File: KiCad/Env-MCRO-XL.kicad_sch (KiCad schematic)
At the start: 49 parts, among them SW1 RotaryEncoder_Switch, SW2 RotaryEncoder_Switch, SW3 RotaryEncoder_Switch, SW4 RotaryEncoder_Switch, U1 Pico

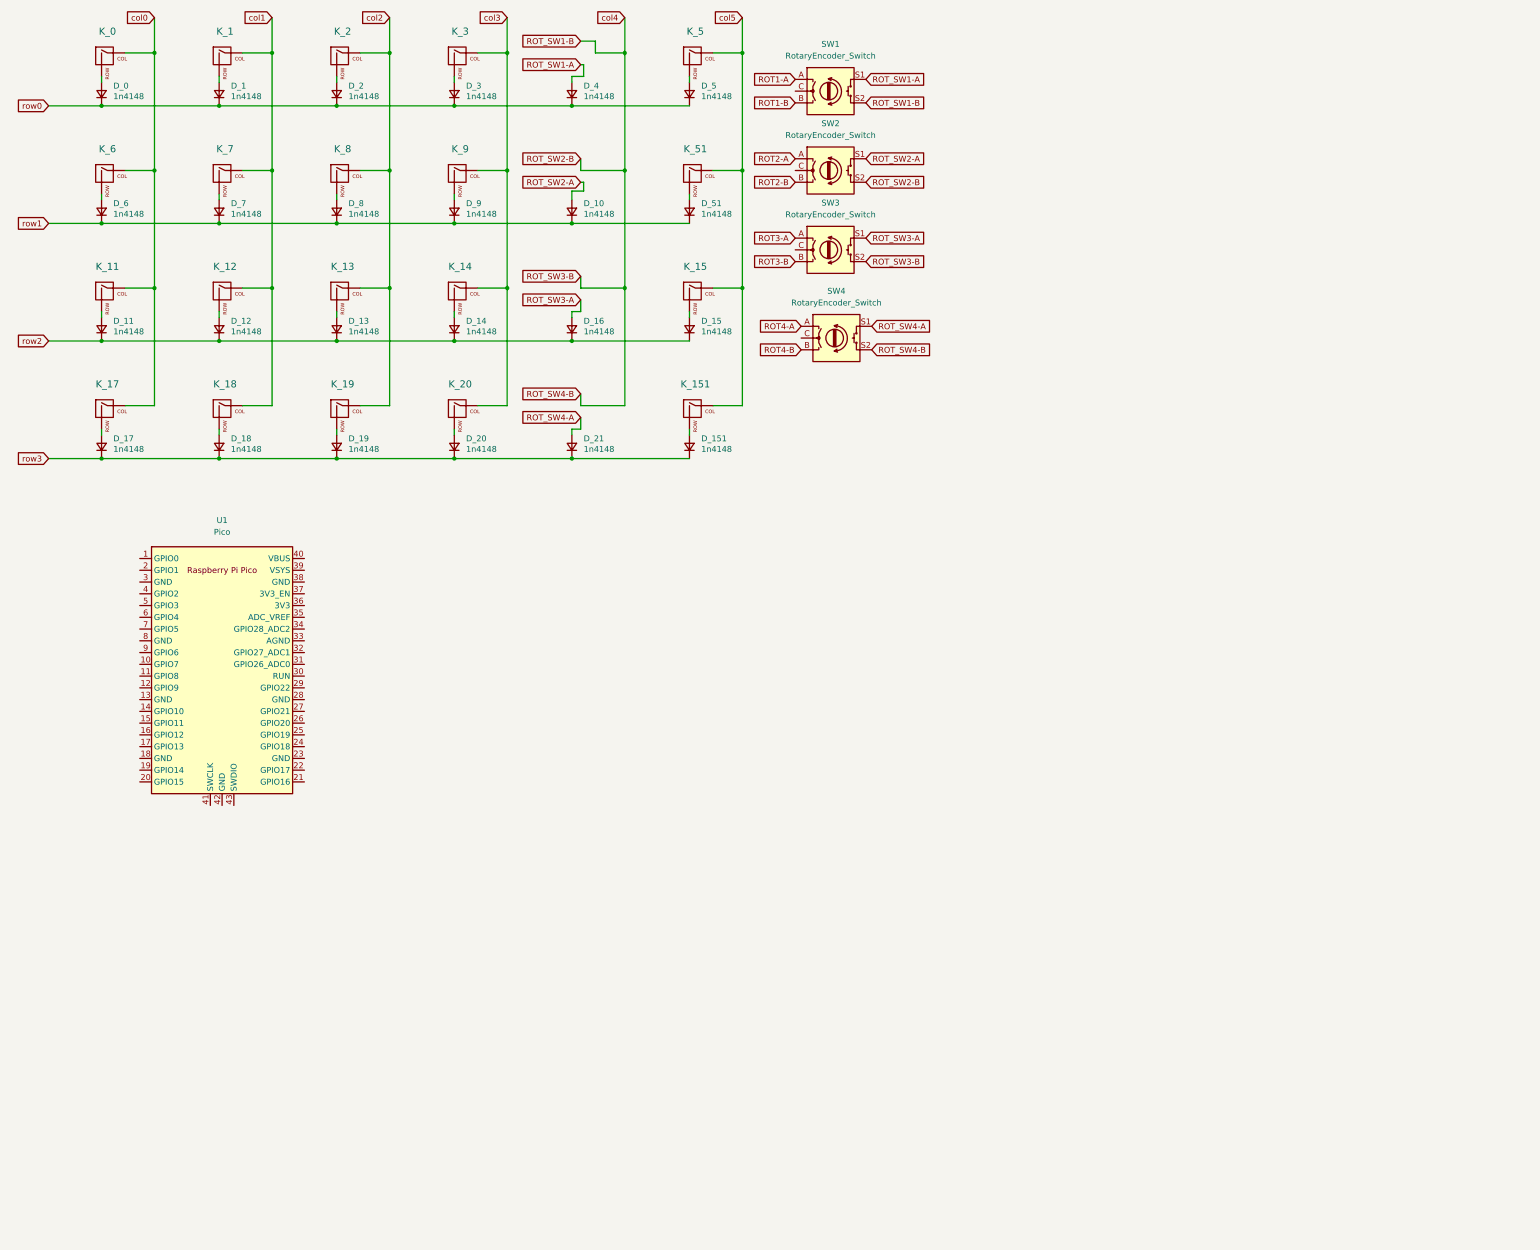
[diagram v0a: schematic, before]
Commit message: Settled on design and wired it up.
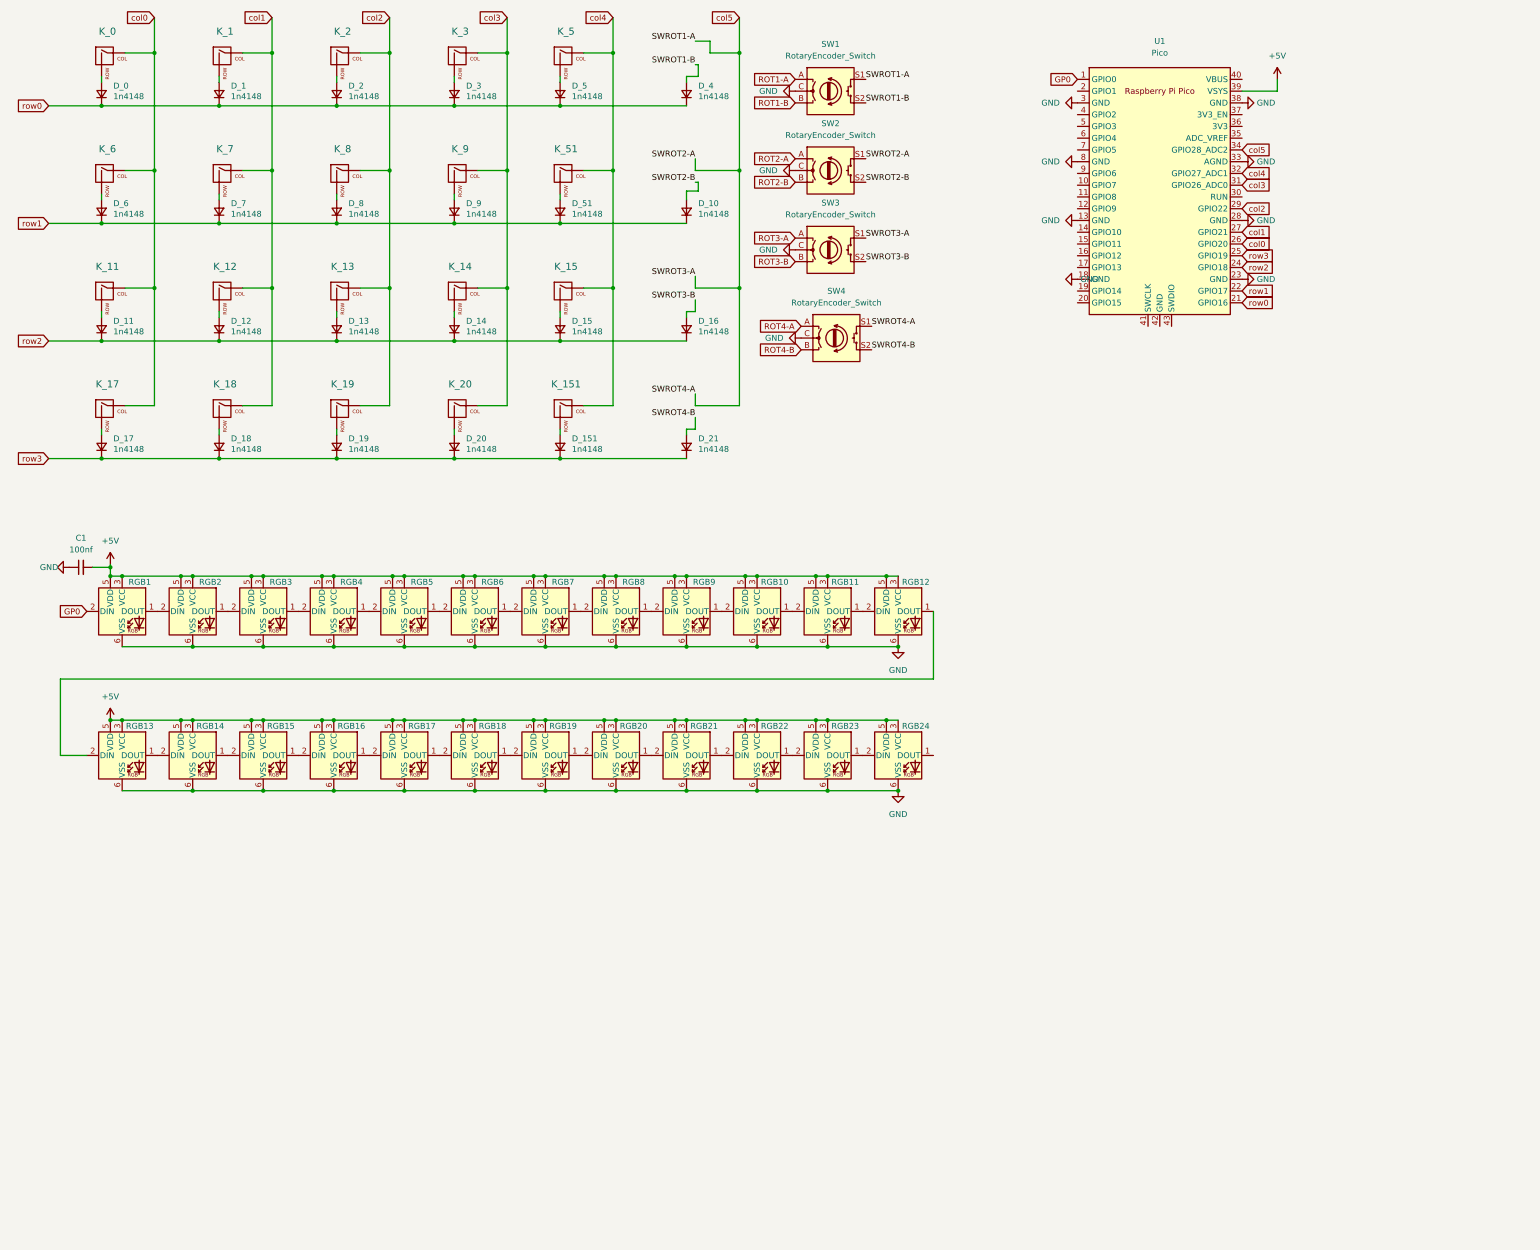
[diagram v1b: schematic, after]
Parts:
- added C1: 100nf, Capacitor_SMD:C_0805_2012Metric, symbol Device:C_Small
- added RGB1, RGB10, RGB11, RGB12, RGB13, RGB14, RGB15, RGB16, RGB17, RGB18, RGB19, RGB2, RGB20, RGB21, RGB22, RGB23, RGB24, RGB3, RGB4, RGB5, RGB6, RGB7, RGB8, RGB9: WS2812, LED_SMD:LED_WS2812_PLCC6_5.0x5.0mm_P1.6mm, symbol LED:WS2812
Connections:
- net col0: now also U1.26 (GPIO20)
- net col1: now also U1.27 (GPIO21)
- net col2: now also U1.29 (GPIO22)
- net col3: now also U1.31 (GPIO26_ADC0)
- net col5: now also SW1.S1, SW2.S1, SW3.S1, SW4.S1, U1.34 (GPIO28_ADC2); no longer K_15.1 (COL), K_151.1 (COL), K_5.1 (COL), K_51.1 (COL)
- net row0: now also U1.21 (GPIO16)
- net row1: now also U1.22 (GPIO17)
- net row2: now also U1.24 (GPIO18)
- net row3: now also U1.25 (GPIO19)
- net GND: now reaches SW3.C
- net GND: now also SW1.C, SW2.C, SW4.C, U1.13 (GND), U1.18 (GND), U1.23 (GND), U1.28 (GND), U1.3 (GND), U1.33 (AGND), U1.38 (GND), U1.8 (GND), C1.1, RGB1.6 (VSS), RGB10.6 (VSS), RGB11.6 (VSS), RGB12.6 (VSS), RGB13.6 (VSS), RGB14.6 (VSS), RGB15.6 (VSS), RGB16.6 (VSS), RGB17.6 (VSS), RGB18.6 (VSS), RGB19.6 (VSS), RGB2.6 (VSS), RGB20.6 (VSS), RGB21.6 (VSS), RGB22.6 (VSS), RGB23.6 (VSS), RGB24.6 (VSS), RGB3.6 (VSS), RGB4.6 (VSS), RGB5.6 (VSS), RGB6.6 (VSS), RGB7.6 (VSS), RGB8.6 (VSS), RGB9.6 (VSS)
- net GP0: now reaches U1.1 (GPIO0)
- net GP0: now also RGB1.2 (DIN)
- net col4: now reaches U1.32 (GPIO27_ADC1)
- net col4: now also K_15.1 (COL), K_151.1 (COL), K_5.1 (COL), K_51.1 (COL)
- net +5V: now reaches U1.39 (VSYS)
- net +5V: now also C1.2, RGB1.3 (VCC), RGB1.5 (VDD), RGB10.3 (VCC), RGB10.5 (VDD), RGB11.3 (VCC), RGB11.5 (VDD), RGB12.3 (VCC), RGB12.5 (VDD), RGB13.3 (VCC), RGB13.5 (VDD), RGB14.3 (VCC), RGB14.5 (VDD), RGB15.3 (VCC), RGB15.5 (VDD), RGB16.3 (VCC), RGB16.5 (VDD), RGB17.3 (VCC), RGB17.5 (VDD), RGB18.3 (VCC), RGB18.5 (VDD), RGB19.3 (VCC), RGB19.5 (VDD), RGB2.3 (VCC), RGB2.5 (VDD), RGB20.3 (VCC), RGB20.5 (VDD), RGB21.3 (VCC), RGB21.5 (VDD), RGB22.3 (VCC), RGB22.5 (VDD), RGB23.3 (VCC), RGB23.5 (VDD), RGB24.3 (VCC), RGB24.5 (VDD), RGB3.3 (VCC), RGB3.5 (VDD), RGB4.3 (VCC), RGB4.5 (VDD), RGB5.3 (VCC), RGB5.5 (VDD), RGB6.3 (VCC), RGB6.5 (VDD), RGB7.3 (VCC), RGB7.5 (VDD), RGB8.3 (VCC), RGB8.5 (VDD), RGB9.3 (VCC), RGB9.5 (VDD)
- net ROT_SW1-A renamed SWROT1-B
- net SWROT1-B: now also SW1.S2; no longer SW1.S1
- removed net ROT_SW1-B: SW1.S2, SW2.S2, SW3.S2, SW4.S2
- net ROT_SW2-A renamed SWROT2-B
- net SWROT2-B: now also SW2.S2; no longer SW2.S1
- net ROT_SW3-A renamed SWROT3-B
- net SWROT3-B: now also SW3.S2; no longer SW3.S1
- net ROT_SW4-A renamed SWROT4-B
- net SWROT4-B: now also SW4.S2; no longer SW4.S1
- new net: RGB21.1 (DOUT), RGB22.2 (DIN)
- new net: RGB20.1 (DOUT), RGB21.2 (DIN)
- new net: RGB10.2 (DIN), RGB9.1 (DOUT)
- new net: RGB8.1 (DOUT), RGB9.2 (DIN)
- new net: RGB23.1 (DOUT), RGB24.2 (DIN)
- new net: RGB17.1 (DOUT), RGB18.2 (DIN)
- new net: RGB16.1 (DOUT), RGB17.2 (DIN)
- new net: RGB4.1 (DOUT), RGB5.2 (DIN)
- new net: RGB3.1 (DOUT), RGB4.2 (DIN)
- new net: RGB14.1 (DOUT), RGB15.2 (DIN)
- new net: RGB13.1 (DOUT), RGB14.2 (DIN)
- new net: RGB10.1 (DOUT), RGB11.2 (DIN)
- new net: RGB12.1 (DOUT), RGB13.2 (DIN)
- new net: RGB7.1 (DOUT), RGB8.2 (DIN)
- new net: RGB6.1 (DOUT), RGB7.2 (DIN)
- new net: RGB5.1 (DOUT), RGB6.2 (DIN)
- new net: RGB18.1 (DOUT), RGB19.2 (DIN)
- new net: RGB19.1 (DOUT), RGB20.2 (DIN)
- new net: RGB11.1 (DOUT), RGB12.2 (DIN)
- new net: RGB2.1 (DOUT), RGB3.2 (DIN)
- new net: RGB1.1 (DOUT), RGB2.2 (DIN)
- new net: RGB15.1 (DOUT), RGB16.2 (DIN)
- new net: RGB22.1 (DOUT), RGB23.2 (DIN)
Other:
- moved on the sheet: D_10, D_15, D_151, D_16, D_21, D_4, D_5, D_51, K_15, K_151, K_5, K_51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

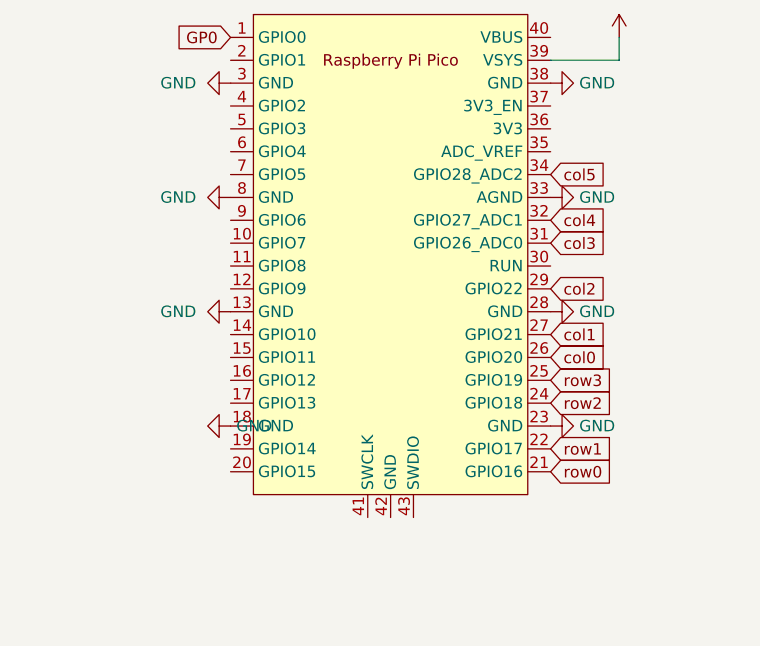
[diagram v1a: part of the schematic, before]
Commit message: various changes and all that.
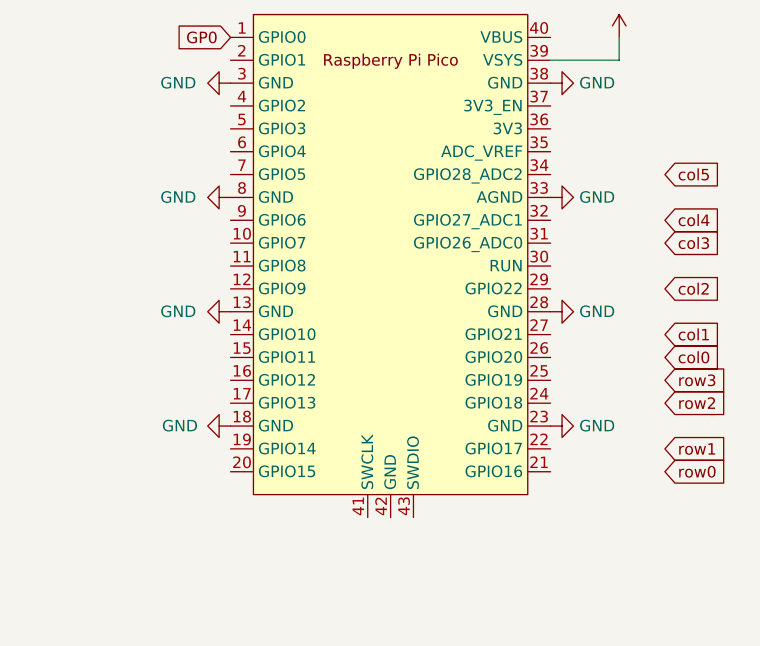
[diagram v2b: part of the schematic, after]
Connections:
- net col0: no longer U1.26 (GPIO20)
- net col1: no longer U1.27 (GPIO21)
- net col2: no longer U1.29 (GPIO22)
- net col3: no longer U1.31 (GPIO26_ADC0)
- net col4: no longer U1.32 (GPIO27_ADC1)
- net col5: no longer U1.34 (GPIO28_ADC2)
- net row0: no longer U1.21 (GPIO16)
- net row1: no longer U1.22 (GPIO17)
- net row2: no longer U1.24 (GPIO18)
- net row3: no longer U1.25 (GPIO19)
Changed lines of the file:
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@@
     )
   )
-  (global_label "col1" (shape input) (at 280.67 62.865 0) (fields_autoplaced)
-    (effects (font (size 1.27 1.27)) (justify left))
-    (property "Intersheet References" "${INTERSHEET_REFS}" (id 0) (at 287.1066 62.7856 0)
+  (global_label "col1" (shape input) (at 293.37 62.865 0) (fields_autoplaced)
+    (effects (font (size 1.27 1.27)) (justify left))
+    (property "Intersheet References" "${INTERSHEET_REFS}" (id 0) (at 299.8066 62.7856 0)
       (effects (font (size 1.27 1.27)) (justify left) hide)
     )
@@
     )
   )
-  (global_label "row1" (shape input) (at 280.67 75.565 0) (fields_autoplaced)
-    (effects (font (size 1.27 1.27)) (justify left))
-    (property "Intersheet References" "${INTERSHEET_REFS}" (id 0) (at 287.4694 75.4856 0)
+  (global_label "row1" (shape input) (at 293.37 75.565 0) (fields_autoplaced)
+    (effects (font (size 1.27 1.27)) (justify left))
+    (property "Intersheet References" "${INTERSHEET_REFS}" (id 0) (at 300.1694 75.4856 0)
       (effects (font (size 1.27 1.27)) (justify left) hide)
     )
@@
     )
   )
-  (global_label "col5" (shape input) (at 280.67 45.085 0) (fields_autoplaced)
-    (effects (font (size 1.27 1.27)) (justify left))
-    (property "Intersheet References" "${INTERSHEET_REFS}" (id 0) (at 287.1066 45.1644 0)
-      (effects (font (size 1.27 1.27)) (justify left) hide)
-    )
-  )
-  (global_label "col0" (shape input) (at 280.67 65.405 0) (fields_autoplaced)
-    (effects (font (size 1.27 1.27)) (justify left))
-    (property "Intersheet References" "${INTERSHEET_REFS}" (id 0) (at 287.1066 65.3256 0)
+  (global_label "col5" (shape input) (at 293.37 45.085 0) (fields_autoplaced)
+    (effects (font (size 1.27 1.27)) (justify left))
+    (property "Intersheet References" "${INTERSHEET_REFS}" (id 0) (at 299.8066 45.1644 0)
+      (effects (font (size 1.27 1.27)) (justify left) hide)
+    )
+  )
+  (global_label "col0" (shape input) (at 293.37 65.405 0) (fields_autoplaced)
+    (effects (font (size 1.27 1.27)) (justify left))
+    (property "Intersheet References" "${INTERSHEET_REFS}" (id 0) (at 299.8066 65.3256 0)
       (effects (font (size 1.27 1.27)) (justify left) hide)
     )
@@
     )
   )
-  (global_label "row2" (shape input) (at 280.67 70.485 0) (fields_autoplaced)
-    (effects (font (size 1.27 1.27)) (justify left))
-    (property "Intersheet References" "${INTERSHEET_REFS}" (id 0) (at 287.4694 70.4056 0)
+  (global_label "row2" (shape input) (at 293.37 70.485 0) (fields_autoplaced)
+    (effects (font (size 1.27 1.27)) (justify left))
+    (property "Intersheet References" "${INTERSHEET_REFS}" (id 0) (at 300.1694 70.4056 0)
       (effects (font (size 1.27 1.27)) (justify left) hide)
     )
@@
     )
   )
-  (global_label "col2" (shape input) (at 280.67 57.785 0) (fields_autoplaced)
-    (effects (font (size 1.27 1.27)) (justify left))
-    (property "Intersheet References" "${INTERSHEET_REFS}" (id 0) (at 287.1066 57.7056 0)
+  (global_label "col2" (shape input) (at 293.37 57.785 0) (fields_autoplaced)
+    (effects (font (size 1.27 1.27)) (justify left))
+    (property "Intersheet References" "${INTERSHEET_REFS}" (id 0) (at 299.8066 57.7056 0)
       (effects (font (size 1.27 1.27)) (justify left) hide)
     )
@@
     )
   )
-  (global_label "col4" (shape input) (at 280.67 50.165 0) (fields_autoplaced)
-    (effects (font (size 1.27 1.27)) (justify left))
-    (property "Intersheet References" "${INTERSHEET_REFS}" (id 0) (at 287.1066 50.0856 0)
-      (effects (font (size 1.27 1.27)) (justify left) hide)
-    )
-  )
-  (global_label "row0" (shape input) (at 280.67 78.105 0) (fields_autoplaced)
-    (effects (font (size 1.27 1.27)) (justify left))
-    (property "Intersheet References" "${INTERSHEET_REFS}" (id 0) (at 287.4694 78.0256 0)
+  (global_label "col4" (shape input) (at 293.37 50.165 0) (fields_autoplaced)
+    (effects (font (size 1.27 1.27)) (justify left))
+    (property "Intersheet References" "${INTERSHEET_REFS}" (id 0) (at 299.8066 50.0856 0)
+      (effects (font (size 1.27 1.27)) (justify left) hide)
+    )
+  )
+  (global_label "row0" (shape input) (at 293.37 78.105 0) (fields_autoplaced)
+    (effects (font (size 1.27 1.27)) (justify left))
+    (property "Intersheet References" "${INTERSHEET_REFS}" (id 0) (at 300.1694 78.0256 0)
       (effects (font (size 1.27 1.27)) (justify left) hide)
     )
@@
     )
   )
-  (global_label "col3" (shape input) (at 280.67 52.705 0) (fields_autoplaced)
-    (effects (font (size 1.27 1.27)) (justify left))
-    (property "Intersheet References" "${INTERSHEET_REFS}" (id 0) (at 287.1066 52.6256 0)
-      (effects (font (size 1.27 1.27)) (justify left) hide)
-    )
-  )
-  (global_label "row3" (shape input) (at 280.67 67.945 0) (fields_autoplaced)
-    (effects (font (size 1.27 1.27)) (justify left))
-    (property "Intersheet References" "${INTERSHEET_REFS}" (id 0) (at 303.53 179.705 0)
+  (global_label "col3" (shape input) (at 293.37 52.705 0) (fields_autoplaced)
+    (effects (font (size 1.27 1.27)) (justify left))
+    (property "Intersheet References" "${INTERSHEET_REFS}" (id 0) (at 299.8066 52.6256 0)
+      (effects (font (size 1.27 1.27)) (justify left) hide)
+    )
+  )
+  (global_label "row3" (shape input) (at 293.37 67.945 0) (fields_autoplaced)
+    (effects (font (size 1.27 1.27)) (justify left))
+    (property "Intersheet References" "${INTERSHEET_REFS}" (id 0) (at 316.23 179.705 0)
       (effects (font (size 1.27 1.27)) hide)
     )
@@
   )
   (symbol (lib_id "power:GND") (at 245.11 73.025 270) (unit 1)
-    (in_bom yes) (on_board yes) (fields_autoplaced)
+    (in_bom yes) (on_board yes)
     (property "Reference" "#PWR0104" (id 0) (at 238.76 73.025 0)
       (effects (font (size 1.27 1.27)) hide)
     )
-    (property "Value" "GND" (id 1) (at 245.745 73.0249 90)
+    (property "Value" "GND" (id 1) (at 237.49 73.025 90)
       (effects (font (size 1.27 1.27)) (justify left))
     )
